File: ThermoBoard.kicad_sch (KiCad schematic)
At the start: 4 parts

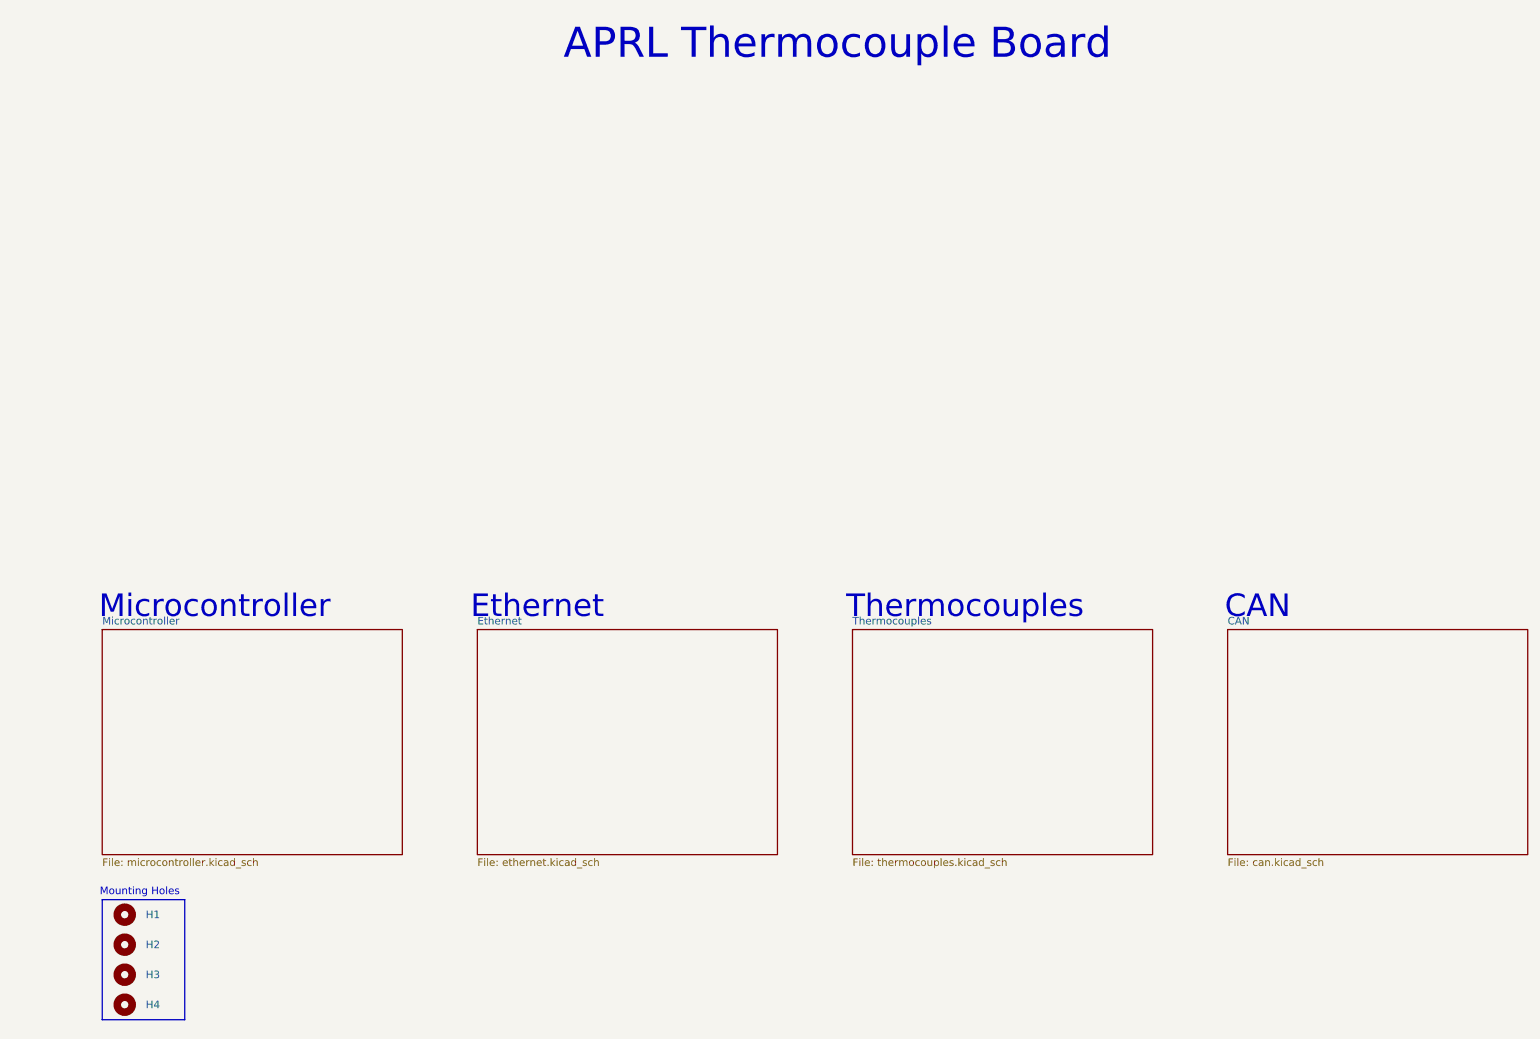
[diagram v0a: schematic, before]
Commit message: First workable layout
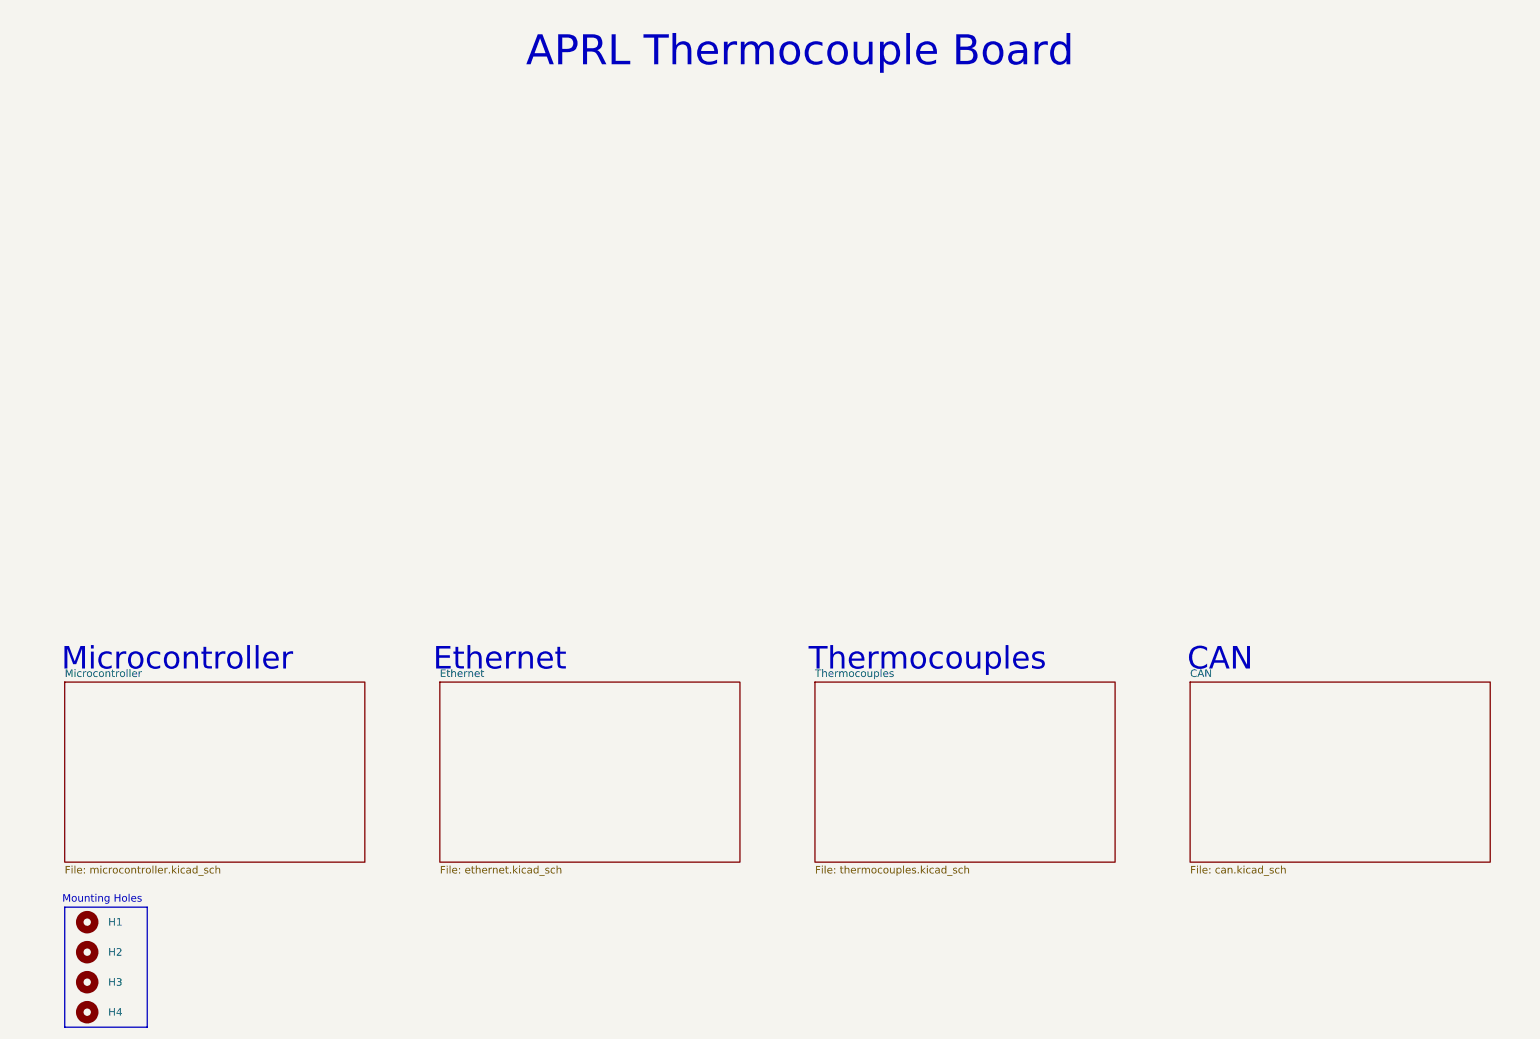
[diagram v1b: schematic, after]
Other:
- moved on the sheet: H1, H2, H3, H4
